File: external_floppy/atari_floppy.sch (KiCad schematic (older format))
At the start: 8 parts, among them J1 12VDC, J2 FLOPPY_PWR, J3 DATA_IN, J4 FLOPPY, U1 L7805

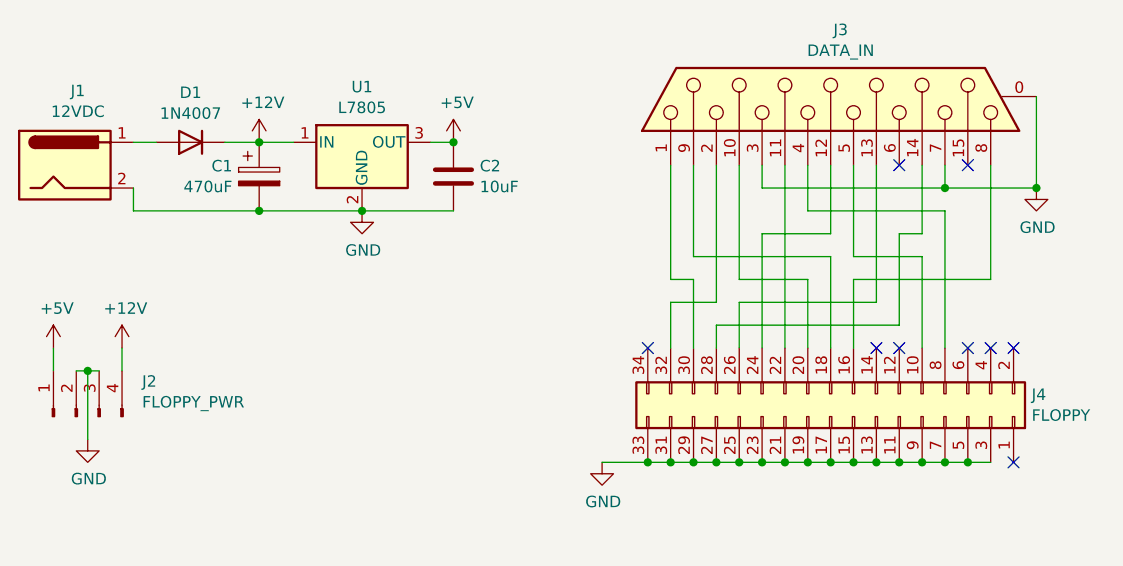
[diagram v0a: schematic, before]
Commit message: a
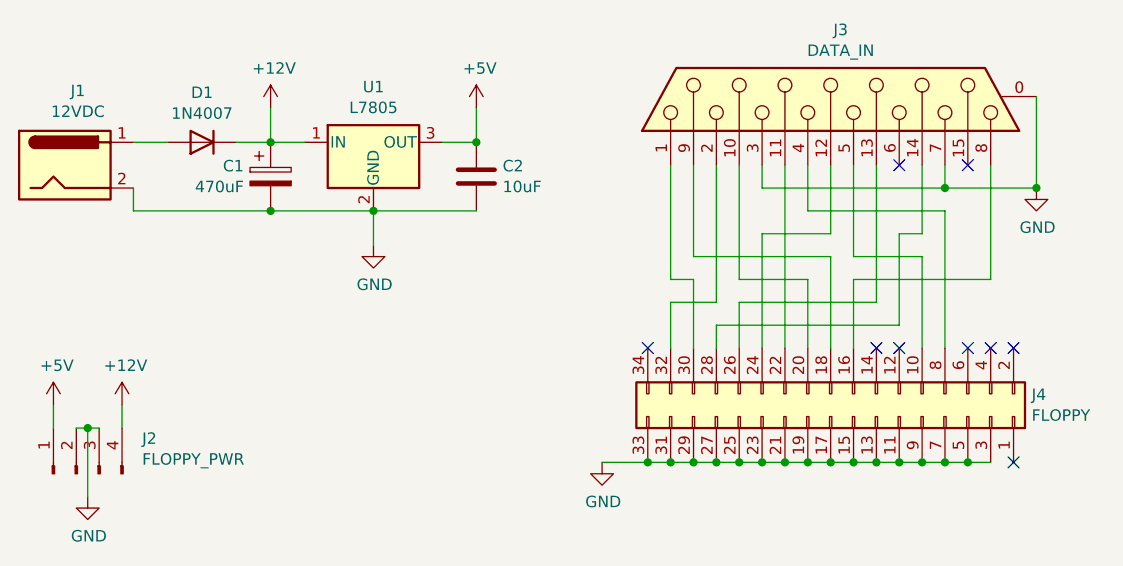
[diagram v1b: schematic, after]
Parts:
- J2: footprint (none) -> atari_floppy:171826-4
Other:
- moved on the sheet: C1, C2, D1, J2, U1
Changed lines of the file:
@@
 Wire Wire Line
 	1400 1550 1400 1450
-Wire Wire Line
-	1500 1250 1400 1250
 $Comp
 L Regulator_Linear:L7812 U1
 U 1 1 5FC363E4
-P 2400 1250
-F 0 "U1" H 2400 1492 50  0000 C CNN
-F 1 "L7805" H 2400 1401 50  0000 C CNN
-F 2 "Package_TO_SOT_THT:TO-220-3_Horizontal_TabDown" H 2425 1100 50  0001 L CIN
-F 3 "http://www.st.com/content/ccc/resource/technical/document/datasheet/41/4f/b3/b0/12/d4/47/88/CD00000444.pdf/files/CD00000444.pdf/jcr:content/translations/en.CD00000444.pdf" H 2400 1200 50  0001 C CNN
-	1    2400 1250
+P 2450 1250
+F 0 "U1" H 2450 1492 50  0000 C CNN
+F 1 "L7805" H 2450 1401 50  0000 C CNN
+F 2 "Package_TO_SOT_THT:TO-220-3_Horizontal_TabDown" H 2475 1100 50  0001 L CIN
+F 3 "http://www.st.com/content/ccc/resource/technical/document/datasheet/41/4f/b3/b0/12/d4/47/88/CD00000444.pdf/files/CD00000444.pdf/jcr:content/translations/en.CD00000444.pdf" H 2450 1200 50  0001 C CNN
+	1    2450 1250
 	1    0    0    -1
 $EndComp
@@
 L Device:C C2
 U 1 1 5FC38FA9
-P 2800 1400
-F 0 "C2" H 2915 1446 50  0000 L CNN
-F 1 "10uF" H 2915 1355 50  0000 L CNN
-F 2 "Capacitor_THT:C_Disc_D10.0mm_W2.5mm_P5.00mm" H 2838 1250 50  0001 C CNN
-F 3 "~" H 2800 1400 50  0001 C CNN
-	1    2800 1400
-	1    0    0    -1
-$EndComp
-Wire Wire Line
-	2800 1250 2700 1250
-Wire Wire Line
-	2800 1550 2400 1550
-Connection ~ 2400 1550
+P 2900 1400
+F 0 "C2" H 3015 1446 50  0000 L CNN
+F 1 "10uF" H 3015 1355 50  0000 L CNN
+F 2 "Capacitor_THT:C_Disc_D10.0mm_W2.5mm_P5.00mm" H 2938 1250 50  0001 C CNN
+F 3 "~" H 2900 1400 50  0001 C CNN
+	1    2900 1400
+	1    0    0    -1
+$EndComp
+Wire Wire Line
+	2900 1250 2750 1250
+Wire Wire Line
+	2900 1550 2450 1550
+Connection ~ 2450 1550
 $Comp
 L power:+5V #PWR06
 U 1 1 5FC3B7C4
-P 2800 1250
-F 0 "#PWR06" H 2800 1100 50  0001 C CNN
-F 1 "+5V" H 2815 1423 50  0000 C CNN
-F 2 "" H 2800 1250 50  0001 C CNN
-F 3 "" H 2800 1250 50  0001 C CNN
-	1    2800 1250
+P 2900 1100
+F 0 "#PWR06" H 2900 950 50  0001 C CNN
+F 1 "+5V" H 2915 1273 50  0000 C CNN
+F 2 "" H 2900 1100 50  0001 C CNN
+F 3 "" H 2900 1100 50  0001 C CNN
+	1    2900 1100
 	1    0    0    -1
 $EndComp
@@
 L power:GND #PWR05
 U 1 1 5FC3C857
-P 2400 1550
-F 0 "#PWR05" H 2400 1300 50  0001 C CNN
-F 1 "GND" H 2405 1377 50  0000 C CNN
-F 2 "" H 2400 1550 50  0001 C CNN
-F 3 "" H 2400 1550 50  0001 C CNN
-	1    2400 1550
+P 2450 1700
+F 0 "#PWR05" H 2450 1450 50  0001 C CNN
+F 1 "GND" H 2455 1527 50  0000 C CNN
+F 2 "" H 2450 1700 50  0001 C CNN
+F 3 "" H 2450 1700 50  0001 C CNN
+	1    2450 1700
 	1    0    0    -1
 $EndComp
@@
 L power:+12V #PWR04
 U 1 1 5FC3F1E7
-P 1950 1250
-F 0 "#PWR04" H 1950 1100 50  0001 C CNN
-F 1 "+12V" H 1965 1423 50  0000 C CNN
-F 2 "" H 1950 1250 50  0001 C CNN
-F 3 "" H 1950 1250 50  0001 C CNN
-	1    1950 1250
+P 2000 1100
+F 0 "#PWR04" H 2000 950 50  0001 C CNN
+F 1 "+12V" H 2015 1273 50  0000 C CNN
+F 2 "" H 2000 1100 50  0001 C CNN
+F 3 "" H 2000 1100 50  0001 C CNN
+	1    2000 1100
 	1    0    0    -1
 $EndComp
@@
 $EndComp
 Wire Wire Line
-	1800 1250 1950 1250
-Wire Wire Line
-	1400 1550 1950 1550
-Connection ~ 1950 1250
-Wire Wire Line
-	1950 1250 2100 1250
-Connection ~ 1950 1550
-Wire Wire Line
-	1950 1550 2400 1550
+	1850 1250 2000 1250
+Connection ~ 2000 1250
+Wire Wire Line
+	2000 1250 2150 1250
+Connection ~ 2000 1550
+Wire Wire Line
+	2000 1550 2450 1550
 $Comp
 L Device:CP C1
 U 1 1 5FC399BB
-P 1950 1400
-F 0 "C1" H 1833 1446 50  0000 R CNN
-F 1 "470uF" H 1833 1355 50  0000 R CNN
-F 2 "Capacitor_THT:C_Radial_D10.0mm_H12.5mm_P5.00mm" H 1988 1250 50  0001 C CNN
-F 3 "~" H 1950 1400 50  0001 C CNN
-	1    1950 1400
+P 2000 1400
+F 0 "C1" H 1883 1446 50  0000 R CNN
+F 1 "470uF" H 1883 1355 50  0000 R CNN
+F 2 "Capacitor_THT:C_Radial_D10.0mm_H12.5mm_P5.00mm" H 2038 1250 50  0001 C CNN
+F 3 "~" H 2000 1400 50  0001 C CNN
+	1    2000 1400
 	1    0    0    -1
 $EndComp
@@
 L Device:D D1
 U 1 1 5FC2CE86
-P 1650 1250
-F 0 "D1" H 1650 1033 50  0000 C CNN
-F 1 "1N4007" H 1650 1124 50  0000 C CNN
-F 2 "Diode_THT:D_DO-41_SOD81_P7.62mm_Horizontal" H 1650 1250 50  0001 C CNN
-F 3 "~" H 1650 1250 50  0001 C CNN
-	1    1650 1250
+P 1700 1250
+F 0 "D1" H 1700 1033 50  0000 C CNN
+F 1 "1N4007" H 1700 1124 50  0000 C CNN
+F 2 "Diode_THT:D_DO-41_SOD81_P7.62mm_Horizontal" H 1700 1250 50  0001 C CNN
+F 3 "~" H 1700 1250 50  0001 C CNN
+	1    1700 1250
 	-1   0    0    1
 $EndComp
-Connection ~ 2800 1250
+Connection ~ 2900 1250
 $Comp
 L Connector:Conn_01x04_Male J2
 U 1 1 5FC54F3F
-P 1150 2450
-F 0 "J2" V 1304 2162 50  0000 R CNN
-F 1 "FLOPPY_PWR" V 1213 2162 50  0000 R CNN
-F 2 "" H 1150 2450 50  0001 C CNN
-F 3 "~" H 1150 2450 50  0001 C CNN
-	1    1150 2450
+P 1150 2700
+F 0 "J2" V 1304 2412 50  0000 R CNN
+F 1 "FLOPPY_PWR" V 1213 2412 50  0000 R CNN
+F 2 "atari_floppy:171826-4" H 1150 2700 50  0001 C CNN
+F 3 "~" H 1150 2700 50  0001 C CNN
+	1    1150 2700
 	0    -1   -1   0
 $EndComp
@@
 L power:GND #PWR02
 U 1 1 5FC570EC
-P 1200 2550
-F 0 "#PWR02" H 1200 2300 50  0001 C CNN
-F 1 "GND" H 1205 2377 50  0000 C CNN
-F 2 "" H 1200 2550 50  0001 C CNN
-F 3 "" H 1200 2550 50  0001 C CNN
-	1    1200 2550
+P 1200 2800
+F 0 "#PWR02" H 1200 2550 50  0001 C CNN
+F 1 "GND" H 1205 2627 50  0000 C CNN
+F 2 "" H 1200 2800 50  0001 C CNN
+F 3 "" H 1200 2800 50  0001 C CNN
+	1    1200 2800
 	1    0    0    -1
 $EndComp
@@
 L power:+12V #PWR03
 U 1 1 5FC5783C
-P 1350 2150
-F 0 "#PWR03" H 1350 2000 50  0001 C CNN
-F 1 "+12V" H 1365 2323 50  0000 C CNN
-F 2 "" H 1350 2150 50  0001 C CNN
-F 3 "" H 1350 2150 50  0001 C CNN
-	1    1350 2150
+P 1350 2400
+F 0 "#PWR03" H 1350 2250 50  0001 C CNN
+F 1 "+12V" H 1365 2573 50  0000 C CNN
+F 2 "" H 1350 2400 50  0001 C CNN
+F 3 "" H 1350 2400 50  0001 C CNN
+	1    1350 2400
 	1    0    0    -1
 $EndComp
@@
 L power:+5V #PWR01
 U 1 1 5FC58019
-P 1050 2150
-F 0 "#PWR01" H 1050 2000 50  0001 C CNN
-F 1 "+5V" H 1065 2323 50  0000 C CNN
-F 2 "" H 1050 2150 50  0001 C CNN
-F 3 "" H 1050 2150 50  0001 C CNN
-	1    1050 2150
-	1    0    0    -1
-$EndComp
-Wire Wire Line
-	1250 2250 1200 2250
-Wire Wire Line
-	1200 2250 1200 2550
-Connection ~ 1200 2250
-Wire Wire Line
-	1200 2250 1150 2250
-Wire Wire Line
-	1350 2250 1350 2150
-Wire Wire Line
-	1050 2250 1050 2150
+P 1050 2400
+F 0 "#PWR01" H 1050 2250 50  0001 C CNN
+F 1 "+5V" H 1065 2573 50  0000 C CNN
+F 2 "" H 1050 2400 50  0001 C CNN
+F 3 "" H 1050 2400 50  0001 C CNN
+	1    1050 2400
+	1    0    0    -1
+$EndComp
+Wire Wire Line
+	1250 2500 1200 2500
+Wire Wire Line
+	1200 2500 1200 2800
+Connection ~ 1200 2500
+Wire Wire Line
+	1200 2500 1150 2500
+Wire Wire Line
+	1350 2500 1350 2400
+Wire Wire Line
+	1050 2500 1050 2400
 $Comp
 L power:GND #PWR08
@@
 NoConn ~ 4650 2150
 NoConn ~ 3650 2150
+Wire Wire Line
+	1400 1250 1550 1250
+Wire Wire Line
+	1400 1550 2000 1550
+Wire Wire Line
+	2900 1100 2900 1250
+Wire Wire Line
+	2000 1250 2000 1100
+Wire Wire Line
+	2450 1550 2450 1700
 $EndSCHEMATC
